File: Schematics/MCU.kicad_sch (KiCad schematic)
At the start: 4 parts, among them U1 ATmega64A-A, Y1 16MHz

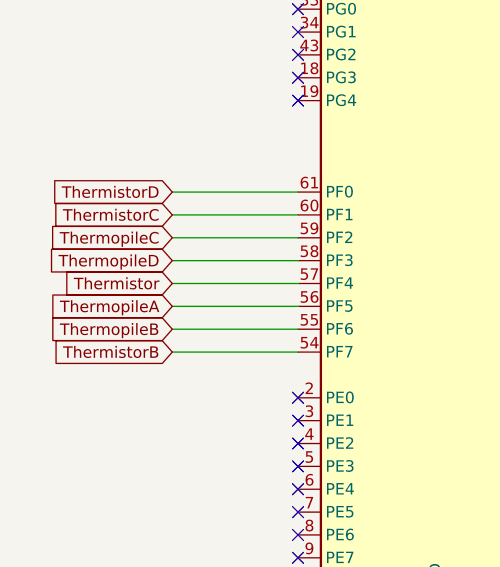
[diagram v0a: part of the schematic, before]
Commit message: Finalized PCB
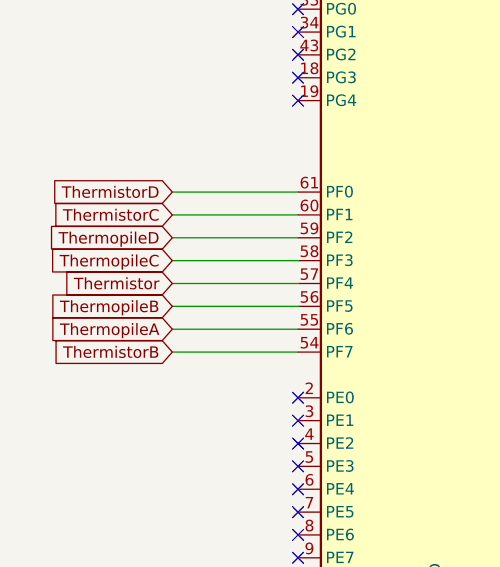
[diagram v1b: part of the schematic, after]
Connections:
- net ThermopileA: now also U1.55 (PF6); no longer U1.56 (PF5)
- net ThermopileB: now also U1.56 (PF5); no longer U1.55 (PF6)
- net ThermopileC: now also U1.58 (PF3); no longer U1.59 (PF2)
- net ThermopileD: now also U1.59 (PF2); no longer U1.58 (PF3)
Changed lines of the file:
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@@
     )
   )
-  (global_label "ThermopileC" (shape input) (at 118.11 111.76 180) (fields_autoplaced)
+  (global_label "ThermopileC" (shape input) (at 118.11 114.3 180) (fields_autoplaced)
     (effects (font (size 1.27 1.27)) (justify right))
-    (property "Intersheet References" "${INTERSHEET_REFS}" (id 0) (at 104.0855 111.8394 0)
+    (property "Intersheet References" "${INTERSHEET_REFS}" (id 0) (at 104.0855 114.3794 0)
       (effects (font (size 1.27 1.27)) (justify right) hide)
     )
@@
     )
   )
-  (global_label "ThermopileB" (shape input) (at 118.11 121.92 180) (fields_autoplaced)
+  (global_label "ThermopileB" (shape input) (at 118.11 119.38 180) (fields_autoplaced)
     (effects (font (size 1.27 1.27)) (justify right))
-    (property "Intersheet References" "${INTERSHEET_REFS}" (id 0) (at 104.0855 121.8406 0)
+    (property "Intersheet References" "${INTERSHEET_REFS}" (id 0) (at 104.0855 119.3006 0)
       (effects (font (size 1.27 1.27)) (justify right) hide)
     )
@@
     )
   )
-  (global_label "ThermopileD" (shape input) (at 118.11 114.3 180) (fields_autoplaced)
+  (global_label "ThermopileD" (shape input) (at 118.11 111.76 180) (fields_autoplaced)
     (effects (font (size 1.27 1.27)) (justify right))
-    (property "Intersheet References" "${INTERSHEET_REFS}" (id 0) (at 104.0855 114.2206 0)
+    (property "Intersheet References" "${INTERSHEET_REFS}" (id 0) (at 104.0855 111.6806 0)
       (effects (font (size 1.27 1.27)) (justify right) hide)
     )
@@
     )
   )
-  (global_label "ThermopileA" (shape input) (at 118.11 119.38 180) (fields_autoplaced)
+  (global_label "ThermopileA" (shape input) (at 118.11 121.92 180) (fields_autoplaced)
     (effects (font (size 1.27 1.27)) (justify right))
-    (property "Intersheet References" "${INTERSHEET_REFS}" (id 0) (at 104.2669 119.4594 0)
+    (property "Intersheet References" "${INTERSHEET_REFS}" (id 0) (at 104.2669 121.9994 0)
       (effects (font (size 1.27 1.27)) (justify right) hide)
     )
